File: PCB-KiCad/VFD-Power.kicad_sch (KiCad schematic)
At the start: 23 parts, among them IC1 74132D, IC2 XL6009, IC3 ZXBM5210, U3 R-78B5.0-2.0

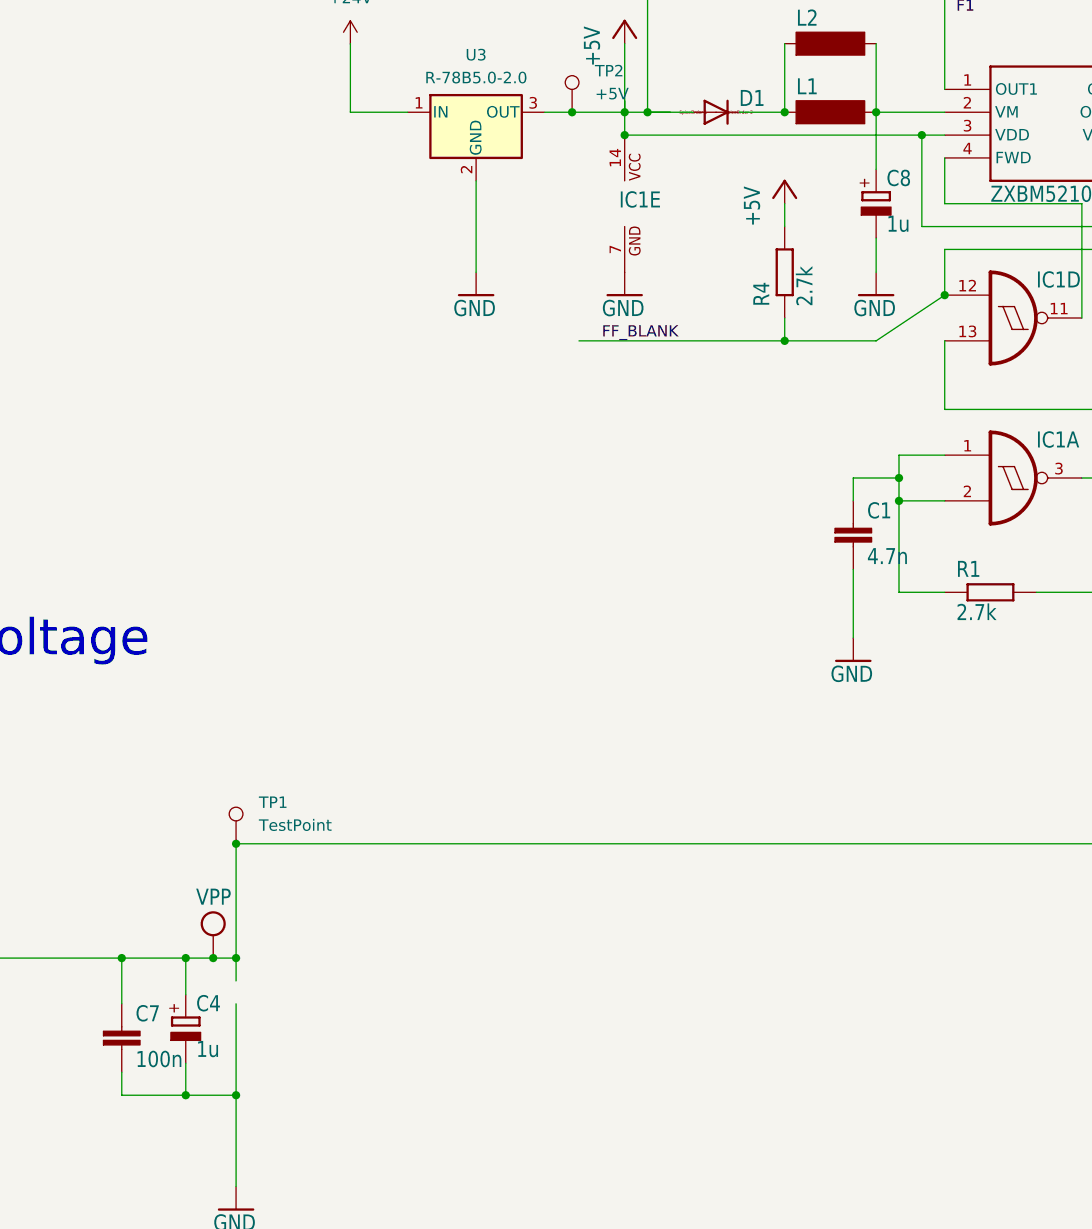
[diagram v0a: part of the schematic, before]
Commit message: Fixed merge issues.
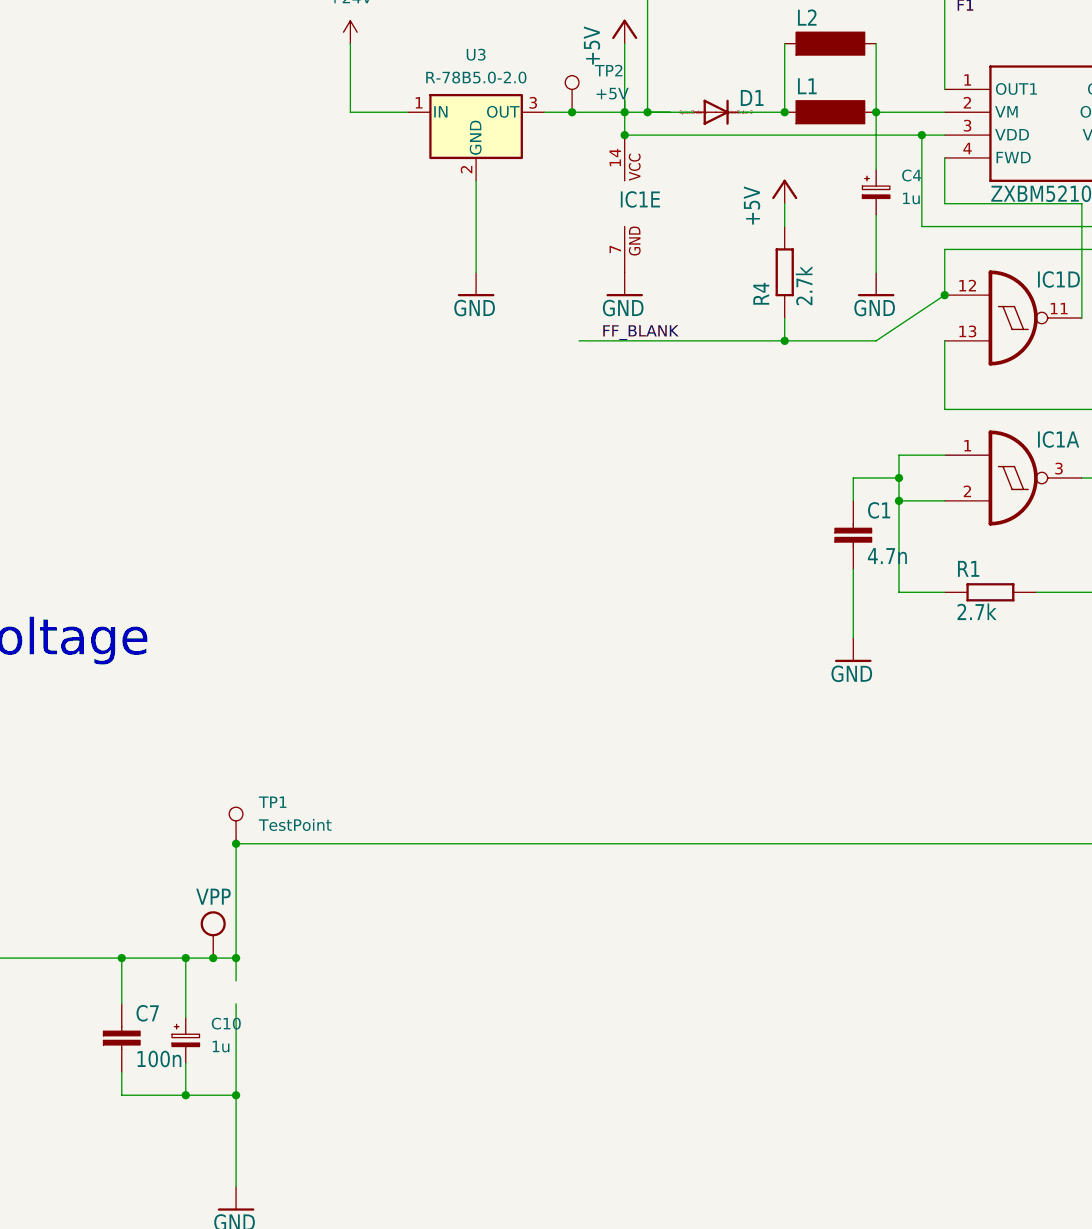
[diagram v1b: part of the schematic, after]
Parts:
- removed C4, C8: 1u, VFD-Power:C1206, symbol VFD-Power-eagle-import:CPOL-EU153CLV-0505
- added C10, C4: 1u, Capacitor_SMD:C_0603_1608Metric_Pad1.08x0.95mm_HandSolder, symbol Device:C_Polarized_Small
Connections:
- net GND: now also C10.2, C4.2
- net VPP: now also C10.1
- net at IC3.2 (VM), L1.2, L2.2: now also C4.1
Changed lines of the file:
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@@
-    (stroke (width 0) (type default))
-  )
-  (wire (pts (xy 112.522 151.384) (xy 112.522 147.32))
     (stroke (width 0) (type default))
   )
@@
     (stroke (width 0.1524) (type solid))
   )
+  (wire (pts (xy 189.23 64.77) (xy 189.23 71.12))
+    (stroke (width 0.1524) (type solid))
+  )
   (wire (pts (xy 179.07 45.72) (xy 179.07 53.34))
     (stroke (width 0.1524) (type solid))
@@
     (stroke (width 0.1524) (type solid))
   )
-  (wire (pts (xy 189.23 71.12) (xy 189.23 67.31))
-    (stroke (width 0.1524) (type solid))
-  )
   (wire (pts (xy 29.21 172.72) (xy 29.21 154.94))
     (stroke (width 0.1524) (type solid))
@@
   (wire (pts (xy 69.85 50.8) (xy 63.5 50.8))
     (stroke (width 0.1524) (type solid))
+  )
+  (wire (pts (xy 112.522 147.32) (xy 112.522 153.924))
+    (stroke (width 0) (type default))
   )
   (wire (pts (xy 130.81 53.34) (xy 137.16 53.34))
@@
         (path "/d66e9896-ee3f-419d-ab82-78a854ae4100"
           (reference "IC3") (unit 1)
-        )
-      )
-    )
-  )
-  (symbol (lib_id "VFD-Power-eagle-import:CPOL-EU153CLV-0505") (at 112.522 153.924 0) (unit 1)
-    (in_bom yes) (on_board yes) (dnp no)
-    (property "Reference" "C4" (at 113.665 153.4414 0)
-      (effects (font (size 1.778 1.5113)) (justify left bottom))
-    )
-    (property "Value" "1u" (at 113.665 158.5214 0)
-      (effects (font (size 1.778 1.5113)) (justify left bottom))
-    )
-    (property "Footprint" "VFD-Power:C1206" (at 112.522 153.924 0)
-      (effects (font (size 1.27 1.27)) hide)
-    )
-    (property "Datasheet" "" (at 112.522 153.924 0)
-      (effects (font (size 1.27 1.27)) hide)
-    )
-    (pin "+")
-    (pin "-")
-    (instances
-      (project "GP1294-Teens4"
-        (path "/3de011e3-f89b-42a8-8637-1f4c3f0867fa/9e049bd2-8c7e-4a7a-b856-b0fbd11ae8df"
-          (reference "C4") (unit 1)
-        )
-      )
-      (project "VFD-Power"
-        (path "/d66e9896-ee3f-419d-ab82-78a854ae4100"
-          (reference "C4") (unit 1)
         )
       )
@@
     )
   )
+  (symbol (lib_id "Device:C_Polarized_Small") (at 189.23 62.23 0) (unit 1)
+    (in_bom yes) (on_board yes) (dnp no) (fields_autoplaced)
+    (property "Reference" "C4" (at 192.024 60.4139 0)
+      (effects (font (size 1.27 1.27)) (justify left))
+    )
+    (property "Value" "1u" (at 192.024 62.9539 0)
+      (effects (font (size 1.27 1.27)) (justify left))
+    )
+    (property "Footprint" "Capacitor_SMD:C_0603_1608Metric_Pad1.08x0.95mm_HandSolder" (at 189.23 62.23 0)
+      (effects (font (size 1.27 1.27)) hide)
+    )
+    (property "Datasheet" "~" (at 189.23 62.23 0)
+      (effects (font (size 1.27 1.27)) hide)
+    )
+    (pin "1")
+    (pin "2")
+    (instances
+      (project "GP1294-Teens4"
+        (path "/3de011e3-f89b-42a8-8637-1f4c3f0867fa/9e049bd2-8c7e-4a7a-b856-b0fbd11ae8df"
+          (reference "C4") (unit 1)
+        )
+      )
+    )
+  )
   (symbol (lib_id "VFD-Power-eagle-import:C-EUC1206") (at 105.41 154.94 0) (unit 1)
     (in_bom yes) (on_board yes) (dnp no)
@@
     )
   )
-  (symbol (lib_id "VFD-Power-eagle-import:CPOL-EU153CLV-0505") (at 189.23 62.23 0) (unit 1)
-    (in_bom yes) (on_board yes) (dnp no)
-    (property "Reference" "C8" (at 190.373 61.7474 0)
-      (effects (font (size 1.778 1.5113)) (justify left bottom))
-    )
-    (property "Value" "1u" (at 190.373 66.8274 0)
-      (effects (font (size 1.778 1.5113)) (justify left bottom))
-    )
-    (property "Footprint" "VFD-Power:C1206" (at 189.23 62.23 0)
-      (effects (font (size 1.27 1.27)) hide)
-    )
-    (property "Datasheet" "" (at 189.23 62.23 0)
-      (effects (font (size 1.27 1.27)) hide)
-    )
-    (pin "+")
-    (pin "-")
-    (instances
-      (project "GP1294-Teens4"
-        (path "/3de011e3-f89b-42a8-8637-1f4c3f0867fa/9e049bd2-8c7e-4a7a-b856-b0fbd11ae8df"
-          (reference "C8") (unit 1)
-        )
-      )
-      (project "VFD-Power"
-        (path "/d66e9896-ee3f-419d-ab82-78a854ae4100"
-          (reference "C8") (unit 1)
-        )
-      )
-    )
-  )
   (symbol (lib_id "VFD-Power-eagle-import:74132D") (at 229.87 93.98 0) (unit 2)
     (in_bom yes) (on_board yes) (dnp no)
@@
         )
       )
+    )
+  )
+  (symbol (lib_id "Device:C_Polarized_Small") (at 112.522 156.464 0) (unit 1)
+    (in_bom yes) (on_board yes) (dnp no) (fields_autoplaced)
+    (property "Reference" "C10" (at 115.316 154.6479 0)
+      (effects (font (size 1.27 1.27)) (justify left))
+    )
+    (property "Value" "1u" (at 115.316 157.1879 0)
+      (effects (font (size 1.27 1.27)) (justify left))
+    )
+    (property "Footprint" "Capacitor_SMD:C_0603_1608Metric_Pad1.08x0.95mm_HandSolder" (at 112.522 156.464 0)
+      (effects (font (size 1.27 1.27)) hide)
+    )
+    (property "Datasheet" "~" (at 112.522 156.464 0)
+      (effects (font (size 1.27 1.27)) hide)
+    )
+    (pin "1")
+    (pin "2")
+    (instances
+      (project "GP1294-Teens4"
+        (path "/3de011e3-f89b-42a8-8637-1f4c3f0867fa/9e049bd2-8c7e-4a7a-b856-b0fbd11ae8df"
+          (reference "C10") (unit 1)
+        )
+      )
